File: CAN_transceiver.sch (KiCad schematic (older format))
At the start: 2 parts, among them U2 SN65HVD233

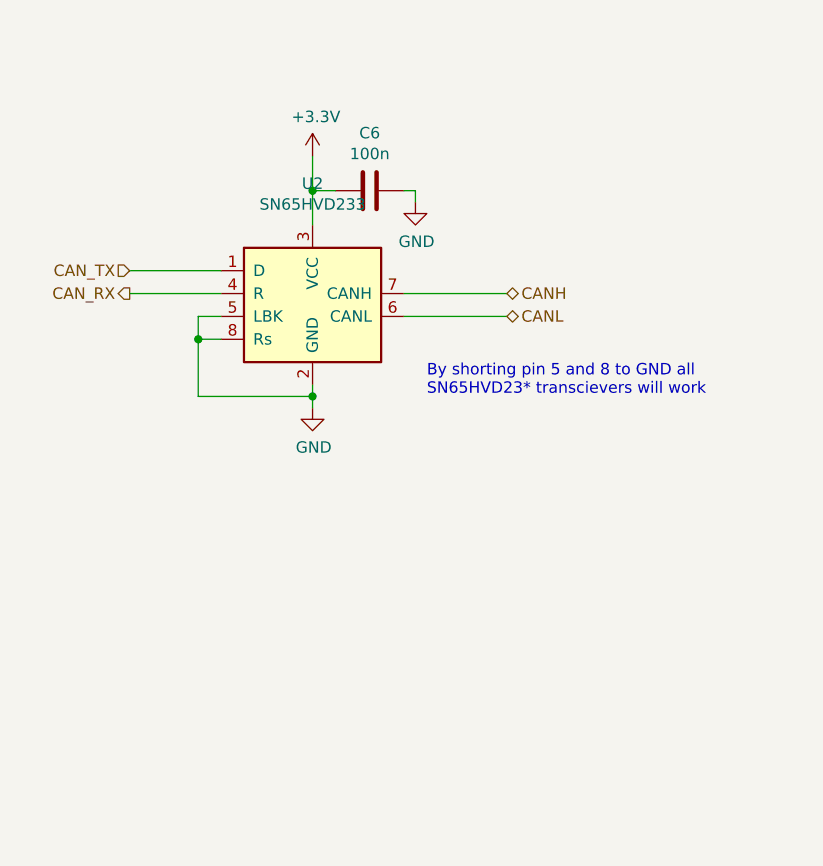
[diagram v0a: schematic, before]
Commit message: Started work on MCU
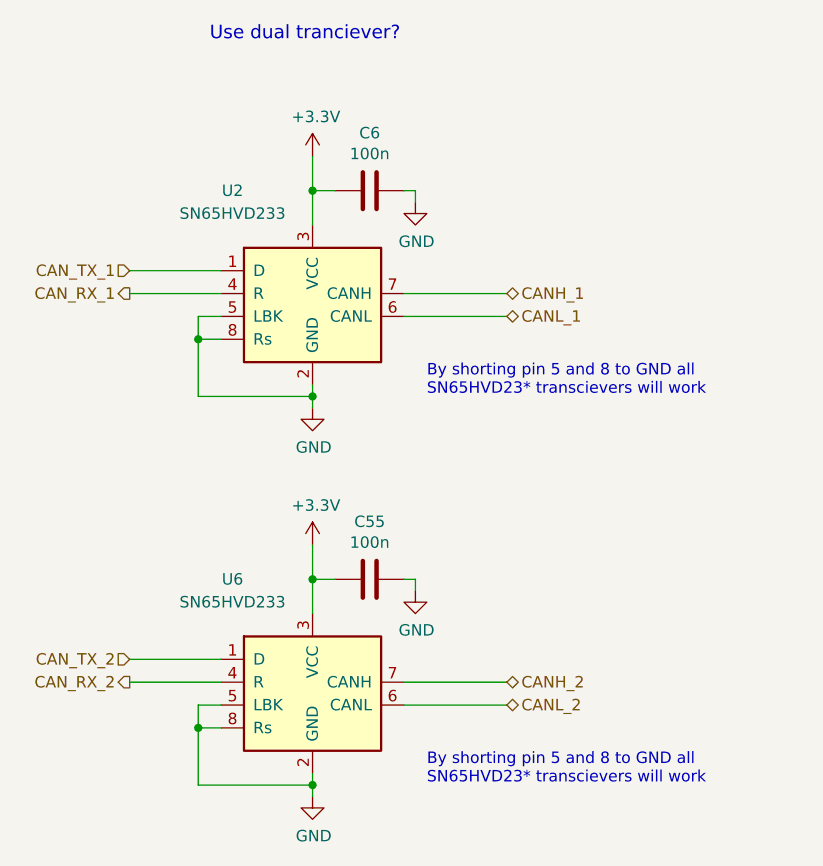
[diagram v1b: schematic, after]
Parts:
- added C55: 100n, symbol Device:C
- added U6: SN65HVD233, Package_SO:SOIC-8_3.9x4.9mm_P1.27mm, symbol Interface_CAN_LIN:SN65HVD233
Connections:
- net +3V3: now also C55.2, U6.3 (VCC)
- net GND: now also C55.1, U6.2 (GND), U6.5 (LBK), U6.8 (Rs)
- net CANH renamed CANH_1
- net CANL renamed CANL_1
- net CAN_RX renamed CAN_RX_1
- net CAN_TX renamed CAN_TX_1
- new net CANH_2: U6.7 (CANH)
- new net CANL_2: U6.6 (CANL)
- new net CAN_RX_2: U6.4 (R)
- new net CAN_TX_2: U6.1 (D)
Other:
- note added: "Use dual tranciever?\n"
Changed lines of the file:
@@
 $EndDescr
 Text HLabel 4700 2900 0    50   Input ~ 0
-CAN_TX
+CAN_TX_1
 Text HLabel 4700 3000 0    50   Output ~ 0
-CAN_RX
+CAN_RX_1
 Wire Wire Line
 	4700 2900 5100 2900
@@
 	5100 3000 4700 3000
 Text HLabel 6350 3000 2    50   BiDi ~ 0
-CANH
+CANH_1
 Text HLabel 6350 3100 2    50   BiDi ~ 0
-CANL
+CANL_1
 Wire Wire Line
 	5900 3000 6350 3000
@@
 U 1 1 5FAEC37C
 P 5500 3000
-F 0 "U2" H 5500 3481 50  0000 C CNN
-F 1 "SN65HVD233" H 5500 3390 50  0000 C CNN
+F 0 "U2" H 5150 3450 50  0000 C CNN
+F 1 "SN65HVD233" H 5150 3350 50  0000 C CNN
 F 2 "Package_SO:SOIC-8_3.9x4.9mm_P1.27mm" H 5500 2500 50  0001 C CNN
 F 3 "http://www.ti.com/lit/ds/symlink/sn65hvd234.pdf" H 5400 3400 50  0001 C CNN
@@
 Text Notes 6000 3450 0    50   ~ 0
 By shorting pin 5 and 8 to GND all\nSN65HVD23* transcievers will work
+Text HLabel 4700 4600 0    50   Input ~ 0
+CAN_TX_2
+Text HLabel 4700 4700 0    50   Output ~ 0
+CAN_RX_2
+Wire Wire Line
+	4700 4600 5100 4600
+Wire Wire Line
+	5100 4700 4700 4700
+Text HLabel 6350 4700 2    50   BiDi ~ 0
+CANH_2
+Text HLabel 6350 4800 2    50   BiDi ~ 0
+CANL_2
+Wire Wire Line
+	5900 4700 6350 4700
+Wire Wire Line
+	6350 4800 5900 4800
+Wire Wire Line
+	5500 4400 5500 4250
+$Comp
+L power:+3.3V #PWR043
+U 1 1 6020E637
+P 5500 4100
+F 0 "#PWR043" H 5500 3950 50  0001 C CNN
+F 1 "+3.3V" H 5515 4273 50  0000 C CNN
+F 2 "" H 5500 4100 50  0001 C CNN
+F 3 "" H 5500 4100 50  0001 C CNN
+	1    5500 4100
+	1    0    0    -1
+$EndComp
+$Comp
+L power:GND #PWR044
+U 1 1 6020E63D
+P 5500 5200
+F 0 "#PWR044" H 5500 4950 50  0001 C CNN
+F 1 "GND" H 5505 5027 50  0000 C CNN
+F 2 "" H 5500 5200 50  0001 C CNN
+F 3 "" H 5500 5200 50  0001 C CNN
+	1    5500 5200
+	1    0    0    -1
+$EndComp
+Wire Wire Line
+	5500 5200 5500 5150
+$Comp
+L Device:C C55
+U 1 1 6020E644
+P 5750 4250
+F 0 "C55" V 5498 4250 50  0000 C CNN
+F 1 "100n" V 5589 4250 50  0000 C CNN
+F 2 "" H 5788 4100 50  0001 C CNN
+F 3 "~" H 5750 4250 50  0001 C CNN
+	1    5750 4250
+	0    1    1    0
+$EndComp
+Wire Wire Line
+	5600 4250 5500 4250
+Connection ~ 5500 4250
+Wire Wire Line
+	5500 4250 5500 4100
+$Comp
+L power:GND #PWR045
+U 1 1 6020E64D
+P 5950 4300
+F 0 "#PWR045" H 5950 4050 50  0001 C CNN
+F 1 "GND" H 5955 4127 50  0000 C CNN
+F 2 "" H 5950 4300 50  0001 C CNN
+F 3 "" H 5950 4300 50  0001 C CNN
+	1    5950 4300
+	1    0    0    -1
+$EndComp
+Wire Wire Line
+	5950 4300 5950 4250
+Wire Wire Line
+	5950 4250 5900 4250
+$Comp
+L Interface_CAN_LIN:SN65HVD233 U6
+U 1 1 6020E655
+P 5500 4700
+F 0 "U6" H 5150 5150 50  0000 C CNN
+F 1 "SN65HVD233" H 5150 5050 50  0000 C CNN
+F 2 "Package_SO:SOIC-8_3.9x4.9mm_P1.27mm" H 5500 4200 50  0001 C CNN
+F 3 "http://www.ti.com/lit/ds/symlink/sn65hvd234.pdf" H 5400 5100 50  0001 C CNN
+	1    5500 4700
+	1    0    0    -1
+$EndComp
+Wire Wire Line
+	5100 4900 5000 4900
+Wire Wire Line
+	5000 5150 5500 5150
+Wire Wire Line
+	5000 4900 5000 5150
+Connection ~ 5500 5150
+Wire Wire Line
+	5500 5150 5500 5100
+Wire Wire Line
+	5100 4800 5000 4800
+Wire Wire Line
+	5000 4800 5000 4900
+Connection ~ 5000 4900
+Text Notes 6000 5150 0    50   ~ 0
+By shorting pin 5 and 8 to GND all\nSN65HVD23* transcievers will work
+Text Notes 5050 1900 0    59   ~ 0
+Use dual tranciever?\n
 $EndSCHEMATC
